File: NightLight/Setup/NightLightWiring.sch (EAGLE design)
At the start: 21 parts

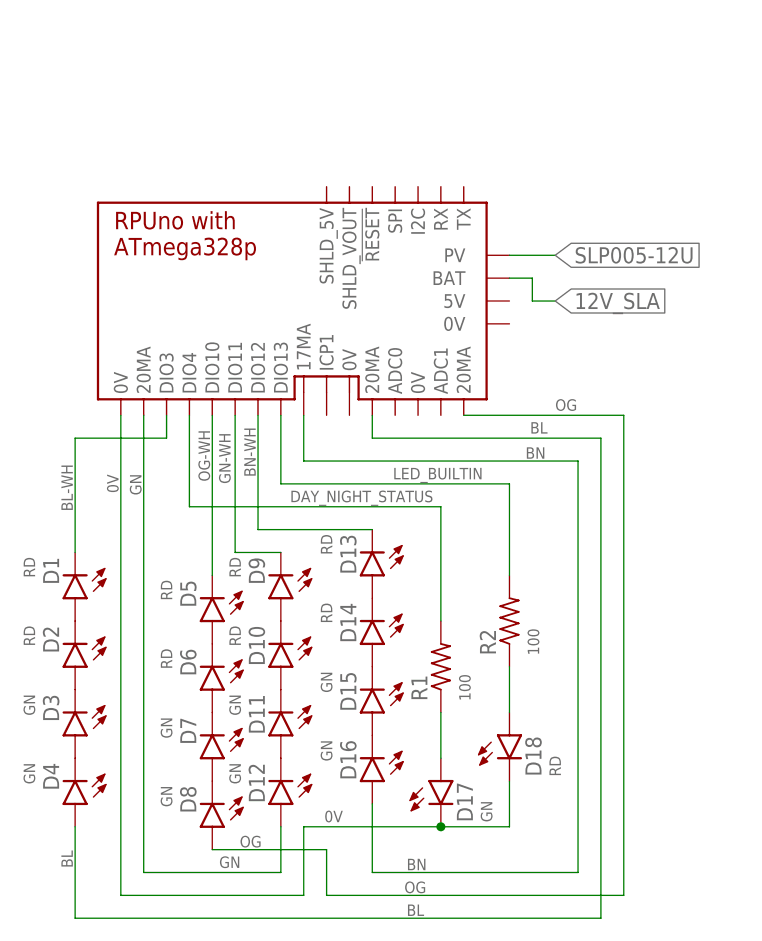
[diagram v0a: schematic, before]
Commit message: NightLight: ^9 updates
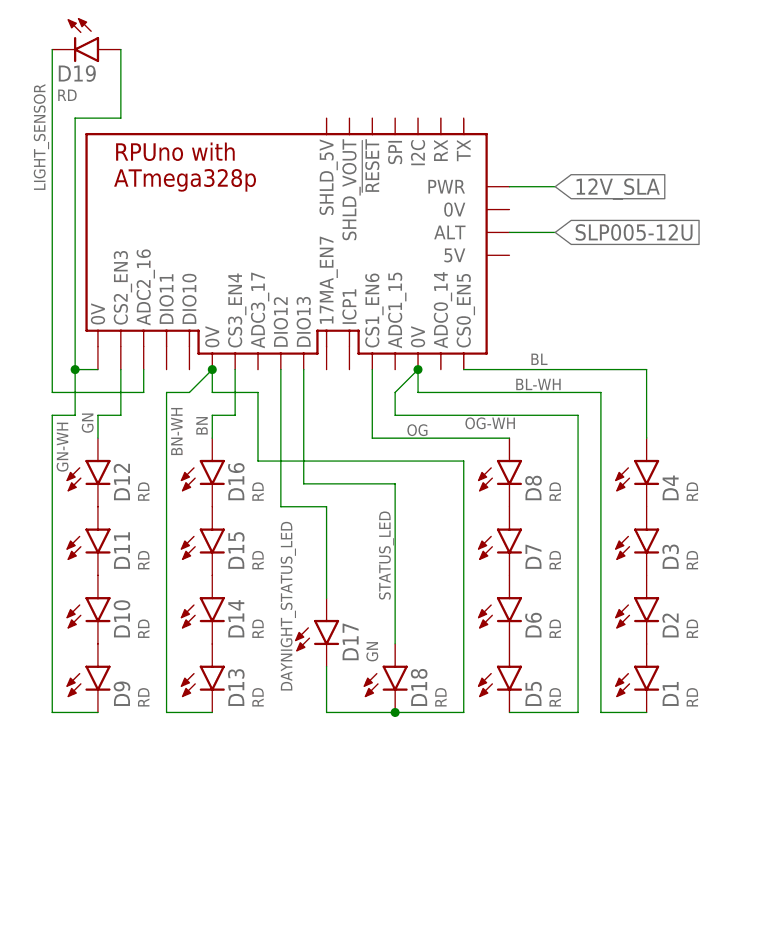
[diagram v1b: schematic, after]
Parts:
- removed R1, R2: 100, R-C:R0805
- added D19: RD, D-LED:LED5MM
- D11, D12, D15, D16, D3, D4, D7, D8: value GN -> RD
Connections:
- removed net DAY_NIGHT_STATUS: BM3.DIO4, R1.2
- removed net LED_BUILTIN: BM3.DIO13, R2.2
- removed net N$1: D17.A, R1.1
- removed net N$2: D18.A, R2.1
- new net DAYNIGHT_STATUS_LED: BM3.DIO12, D17.A
- new net LIGHT_SENSOR: BM3.ADC2_16, D19.K
- new net STATUS_LED: BM3.DIO13, D18.A
- net 0V: no longer BM3.0V@3
- net 12V_SLA: now also BM3.PWR; no longer BM3.BAT
- net BL: now also BM3.CS0_EN5; no longer BM3.20MA@0
- net BL-WH: now also BM3.0V@3; no longer BM3.DIO3
- net BN: now also BM3.CS3_EN4; no longer BM3.17MA@0
- net BN-WH: now also BM3.0V@6; no longer BM3.DIO12
- net GN: now also BM3.CS2_EN3; no longer BM3.20MA@2
- net GN-WH: now also BM3.0V@5, D19.A; no longer BM3.DIO11
- net OG: now also BM3.CS1_EN6; no longer BM3.20MA@1
- net OG-WH: no longer BM3.DIO10
- net SLP005-12U: now also BM3.ALT; no longer BM3.PV
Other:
- moved on the sheet: D1, D10, D11, D12, D13, D14, D15, D16, D17, D18, D2, D3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
